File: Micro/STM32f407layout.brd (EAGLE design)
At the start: 36 x 73 mm, 43 parts, among them Q1 ASF, U1 LM1085IS-3.3

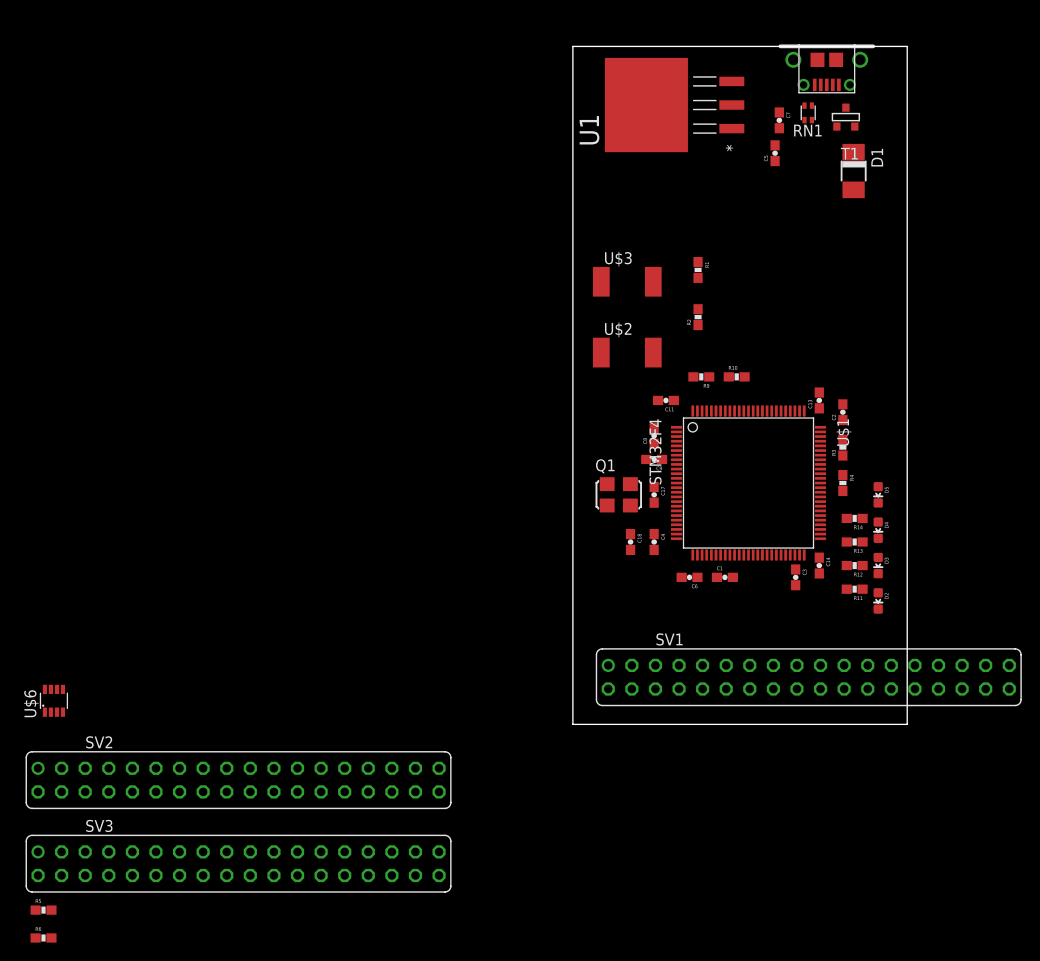
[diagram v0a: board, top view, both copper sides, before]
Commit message: Updated Board
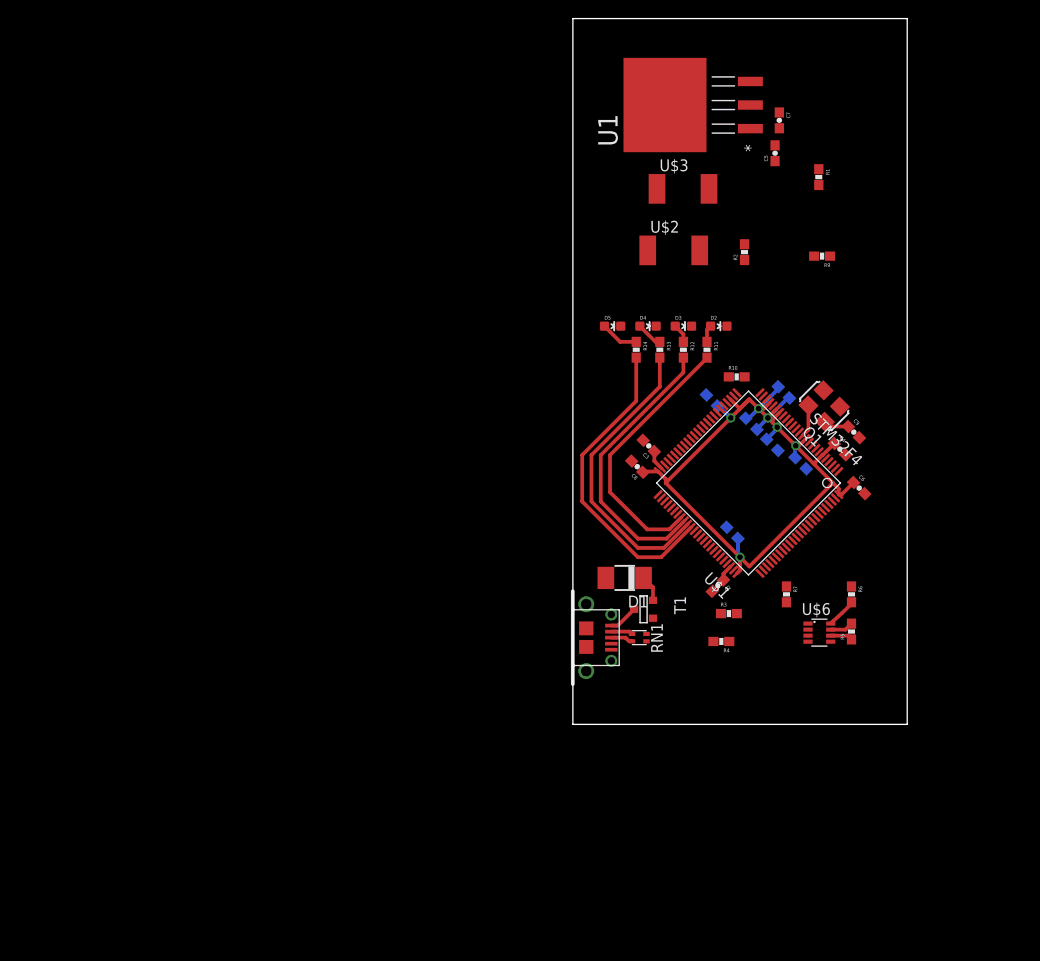
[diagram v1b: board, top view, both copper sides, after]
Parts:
- removed SV1, SV2, SV3: (no value), Connectors:FE18-2
- added R7: 4.7K, SparkFun-Passives:0603-RES
- moved R6 94.5 mm to (30.0, 14.0), turned to 270 degrees
- moved R5 92.0 mm to (30.0, 10.0), turned to 90 degrees
- moved U$6 82.7 mm to (26.5, 9.88), turned to 270 degrees
- moved U$4 69.3 mm to (-0.01, 9.34), turned to 270 degrees
- moved RN1 59.4 mm to (7.15, 9.34), turned to 270 degrees
- moved T1 57.3 mm to (7.61, 12.4), turned to 270 degrees
- moved D1 50.3 mm to (5.58, 15.8), turned to 180 degrees
- moved D2 34.2 mm to (15.7, 42.9), turned to 270 degrees
- moved D5 33.9 mm to (4.28, 42.9), turned to 270 degrees
- moved D3 33.2 mm to (11.9, 42.9), turned to 270 degrees
- moved D4 33.1 mm to (8.09, 42.9), turned to 270 degrees
- moved R11 30.3 mm to (14.4, 40.3), turned to 270 degrees
- moved R14 29.7 mm to (6.82, 40.3), turned to 270 degrees
- moved R12 29.7 mm to (11.9, 40.3), turned to 270 degrees
- moved R13 29.5 mm to (9.36, 40.3), turned to 270 degrees
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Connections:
- removed net CAN1_RX: SV1.1
- removed net CAN1_TX: SV1.3
- new net TEMP_SENSE_INFO: R7.1, U$1.P81
- net +3V3: now also R7.2; no longer SV1.4
- net +5V: no longer SV1.2
- net CAN2_RX: no longer SV1.5
- net CAN2_TX: no longer SV1.7
- net GND: no longer SV1.12, SV1.6, SV1.8
- net I2C1_SCL: no longer SV1.33
- net I2C1_SDA: no longer SV1.35
- net I2C3_SCL: no longer SV1.17
- net I2C3_SDA: no longer SV1.19
- net OSC_IN: no longer SV1.15
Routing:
- net +3V3: track 0.00 -> 84.9 mm, vias 0 -> 5
- net N$9: track 0.00 -> 33.4 mm
- net N$16: track 0.00 -> 32.0 mm
- net N$8: track 0.00 -> 30.6 mm
- net N$19: track 0.00 -> 28.7 mm
- net N$22: track 0.00 -> 6.27 mm, vias 0 -> 1
- net N$15: track 0.00 -> 4.12 mm
- net OSC_IN: track 0.00 -> 3.49 mm
- net N$11: track 0.00 -> 3.46 mm
- net N$10: track 0.00 -> 3.18 mm
- net N$17: track 0.00 -> 2.85 mm
- net N$5: track 0.00 -> 2.83 mm
- net CANH1: track 0.00 -> 2.50 mm
- net CANL1: track 0.00 -> 2.40 mm
- net N$6: track 0.00 -> 2.40 mm
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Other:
- board size 36 x 73 mm -> 36 x 76 mm
